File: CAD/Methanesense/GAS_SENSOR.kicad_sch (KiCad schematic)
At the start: 15 parts, among them Q1 FDS6898A, U2 ADS1115IDGS

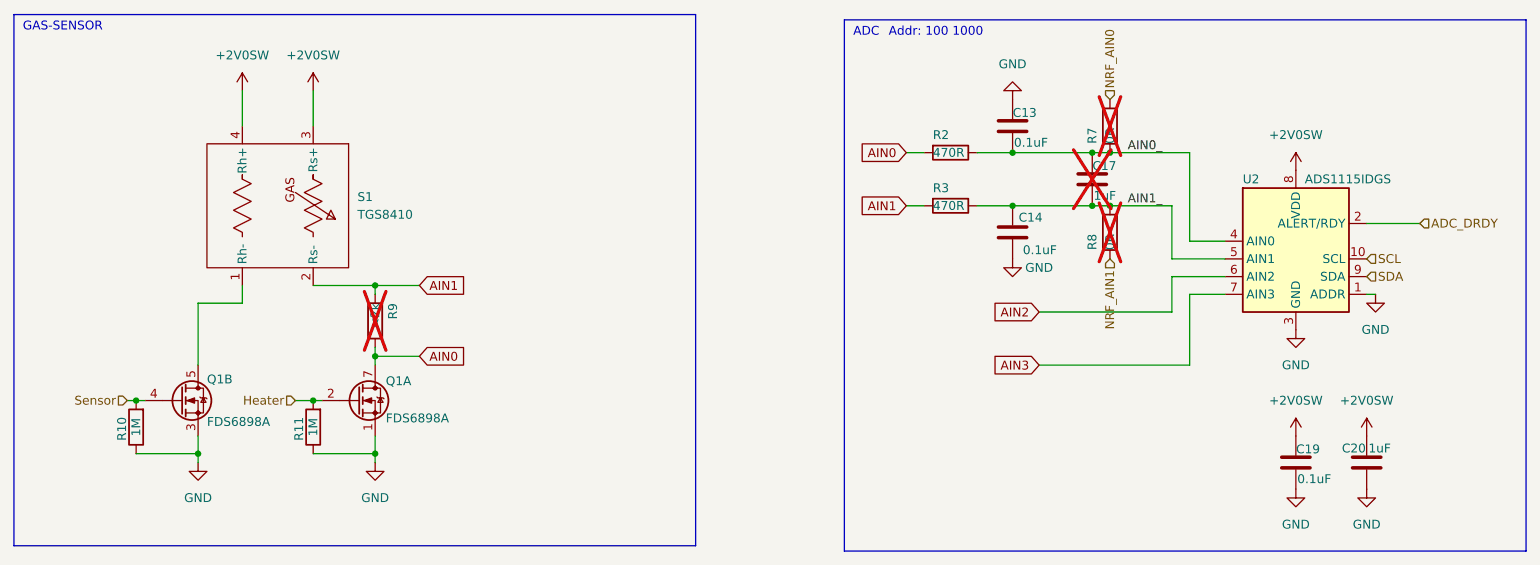
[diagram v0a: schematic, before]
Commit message: rev 1.2
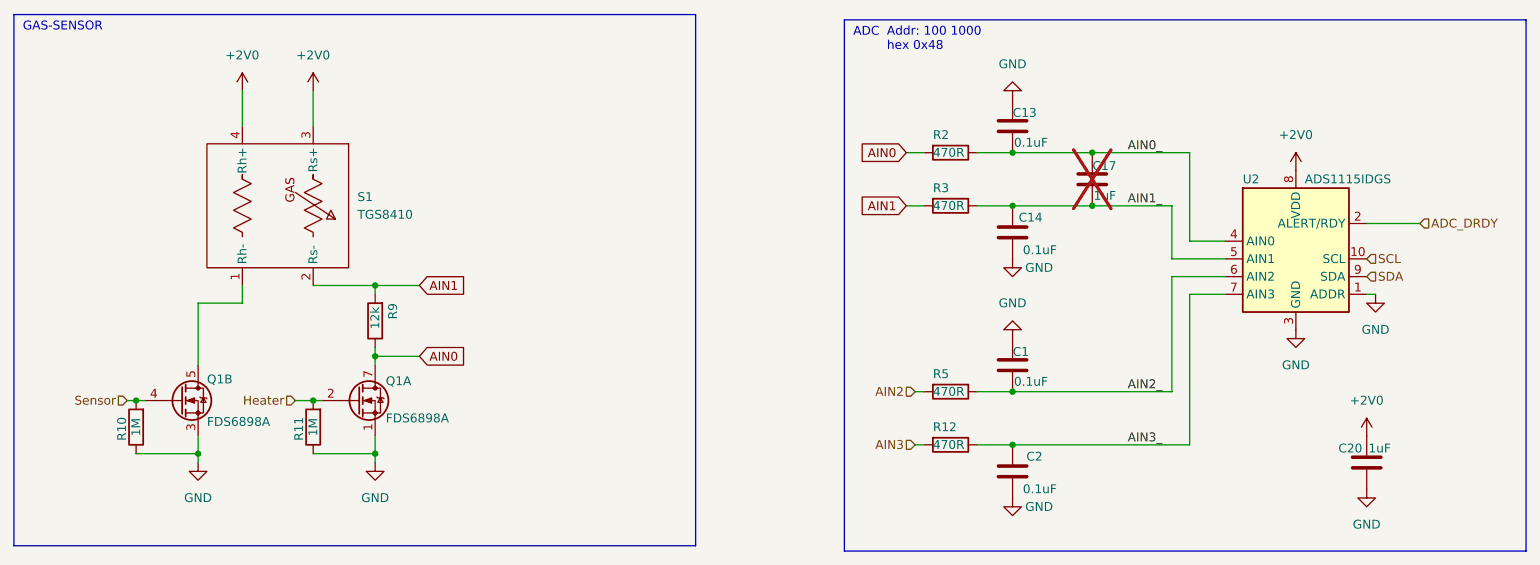
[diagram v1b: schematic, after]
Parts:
- removed C19: 0.1uF, Capacitor_SMD:C_0603_1608Metric, symbol Library:C
- removed R7, R8: 0R, Resistor_SMD:R_0603_1608Metric, symbol Library:R
- added C1, C2: 0.1uF, Capacitor_SMD:C_0603_1608Metric, symbol Library:C
- added R12, R5: 470R, Resistor_SMD:R_0603_1608Metric, symbol Library:R
- R9: value <2k -> 12k; now fitted
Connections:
- net AIN2: now also R5.2; no longer U2.6 (AIN2)
- net AIN3: now also R12.2; no longer U2.7 (AIN3)
- net GND: now also C1.1, C2.1
- net +2V0SW renamed +2V0
- new net AIN2_: C1.2, R5.1, U2.6 (AIN2)
- new net AIN3_: C2.2, R12.1, U2.7 (AIN3)
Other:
- note added: "Addr: 100 1000 hex 0x48"
- note removed: "Addr: 100 1000"
